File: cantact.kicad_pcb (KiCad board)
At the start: 2 copper layers, 36.1 x 59.9 mm, 40 parts, among them J1 Cantact, P2 SWD, P4 USB_C_Plug_USB2.0, U1 STM32F042C6T6, U3 MCP2551-I/SN, U4 XC6220B331MR-G, Y1 16 Mhz

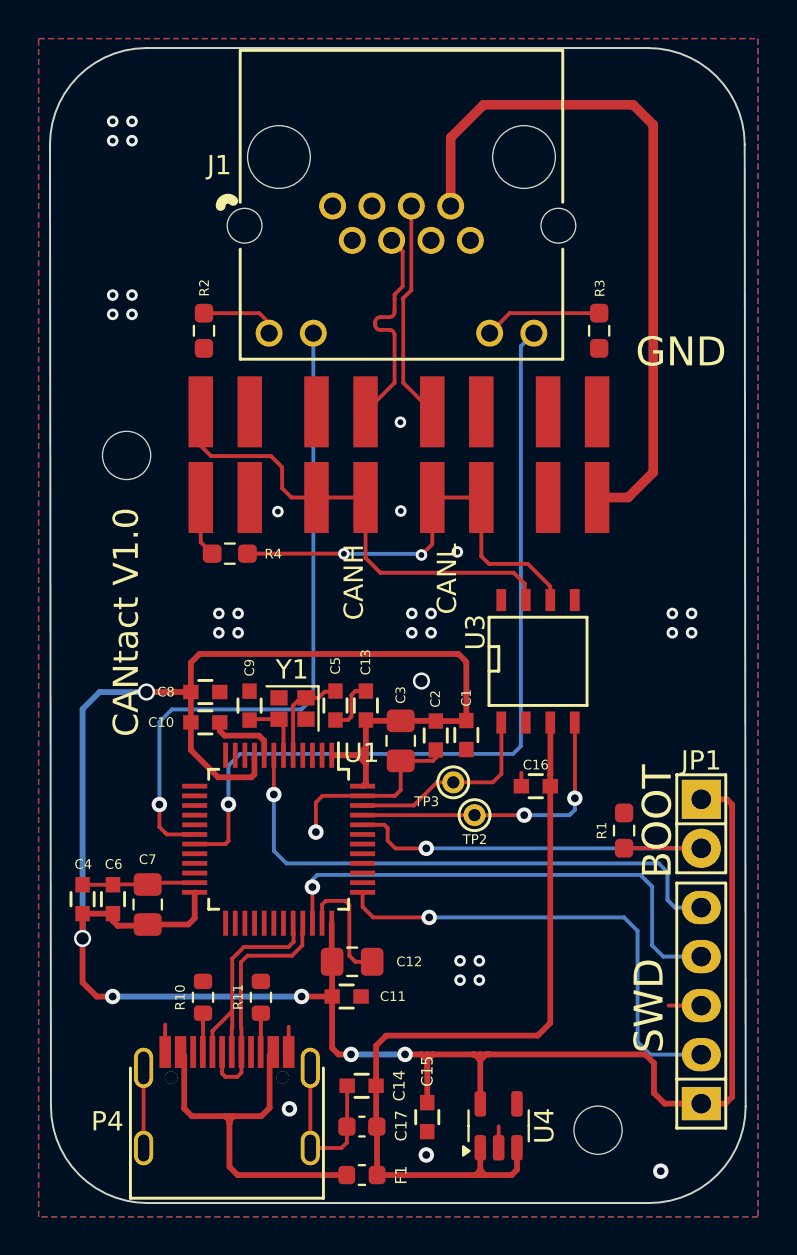
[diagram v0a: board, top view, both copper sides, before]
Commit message: feat(hw): update pcb
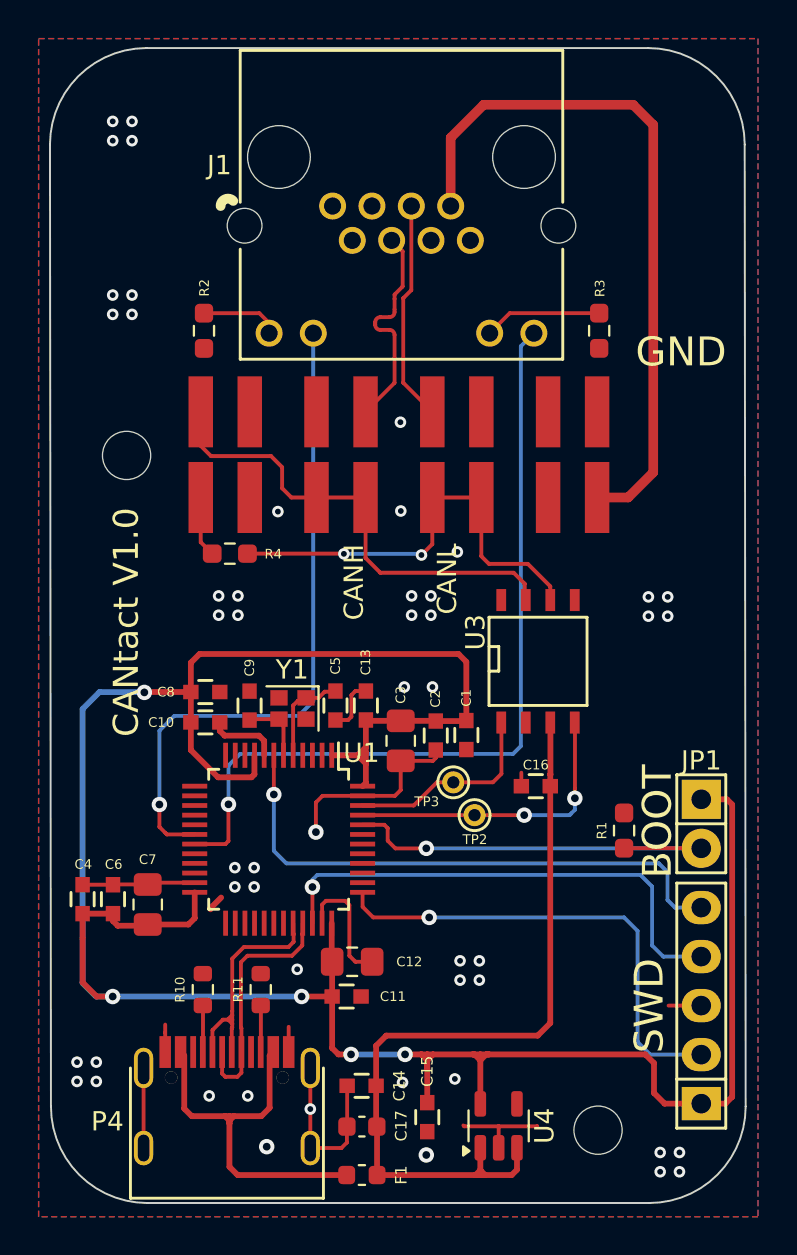
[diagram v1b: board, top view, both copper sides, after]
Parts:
- moved R10 0.40 mm to (132.2, 141.0)
- moved R11 0.40 mm to (135.2, 141.0)
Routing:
- net GND: track 48.7 -> 53.4 mm, vias 33 -> 51
- net +3V3: track 135.2 -> 139.5 mm, vias 6 -> 5
